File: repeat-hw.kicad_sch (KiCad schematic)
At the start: 39 parts, among them J1 USB_C_Receptacle_USB2.0, U1 nRF5340-QKxx, U2 USBLC6-2SC6, Y1 32MHz

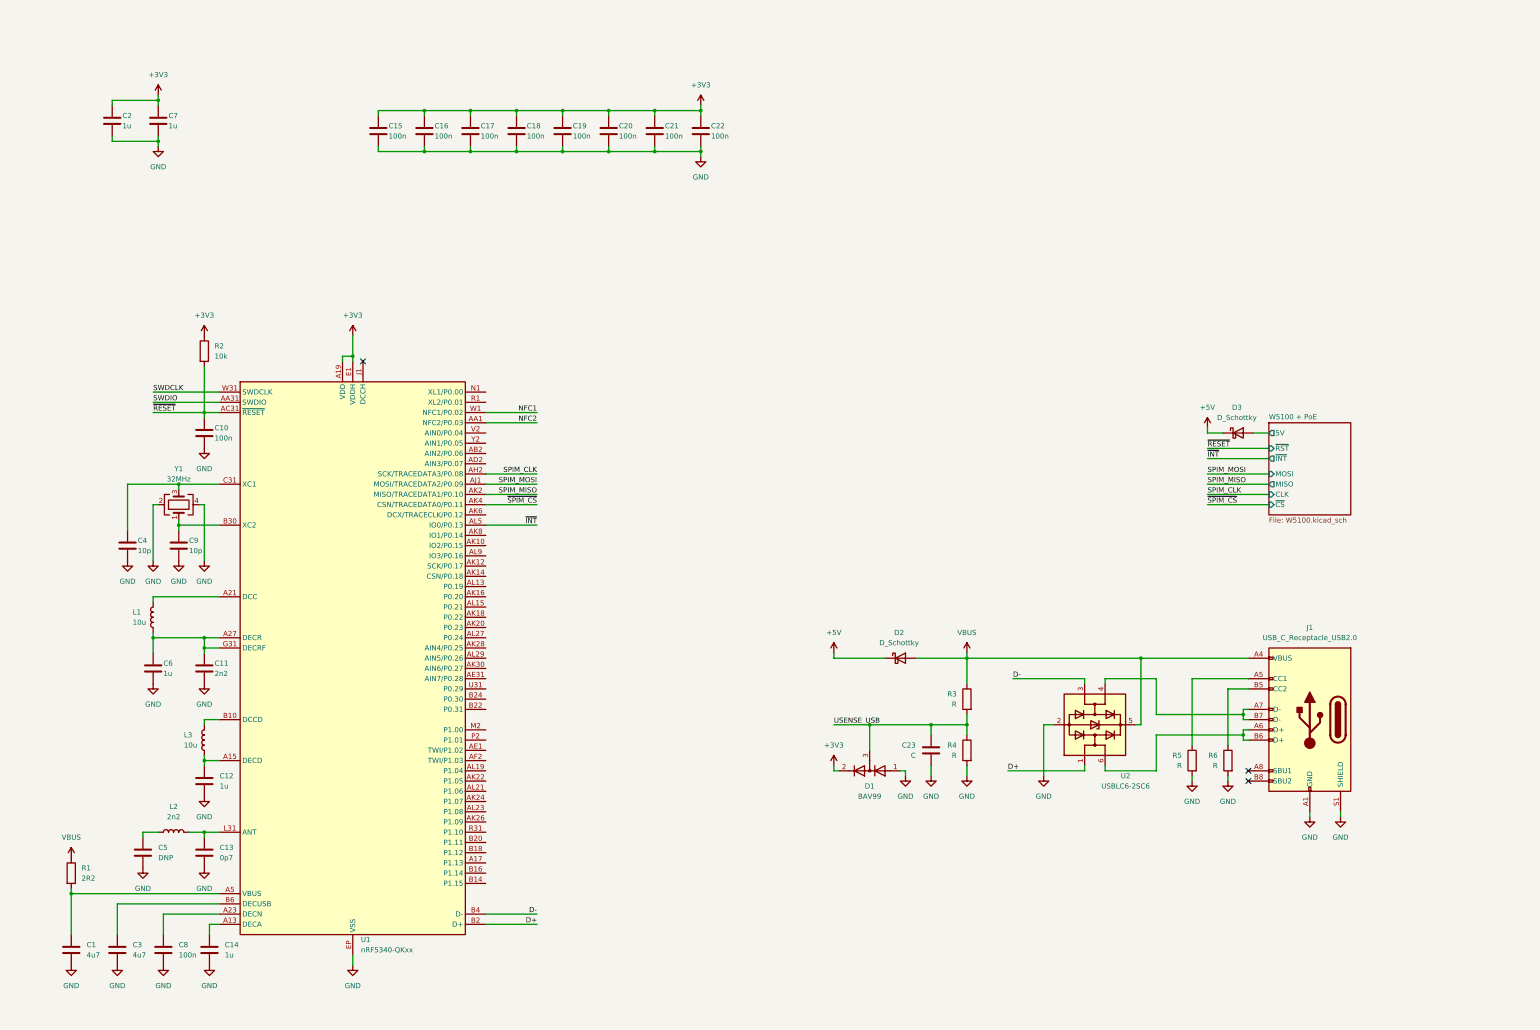
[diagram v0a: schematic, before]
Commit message: Polished schematic
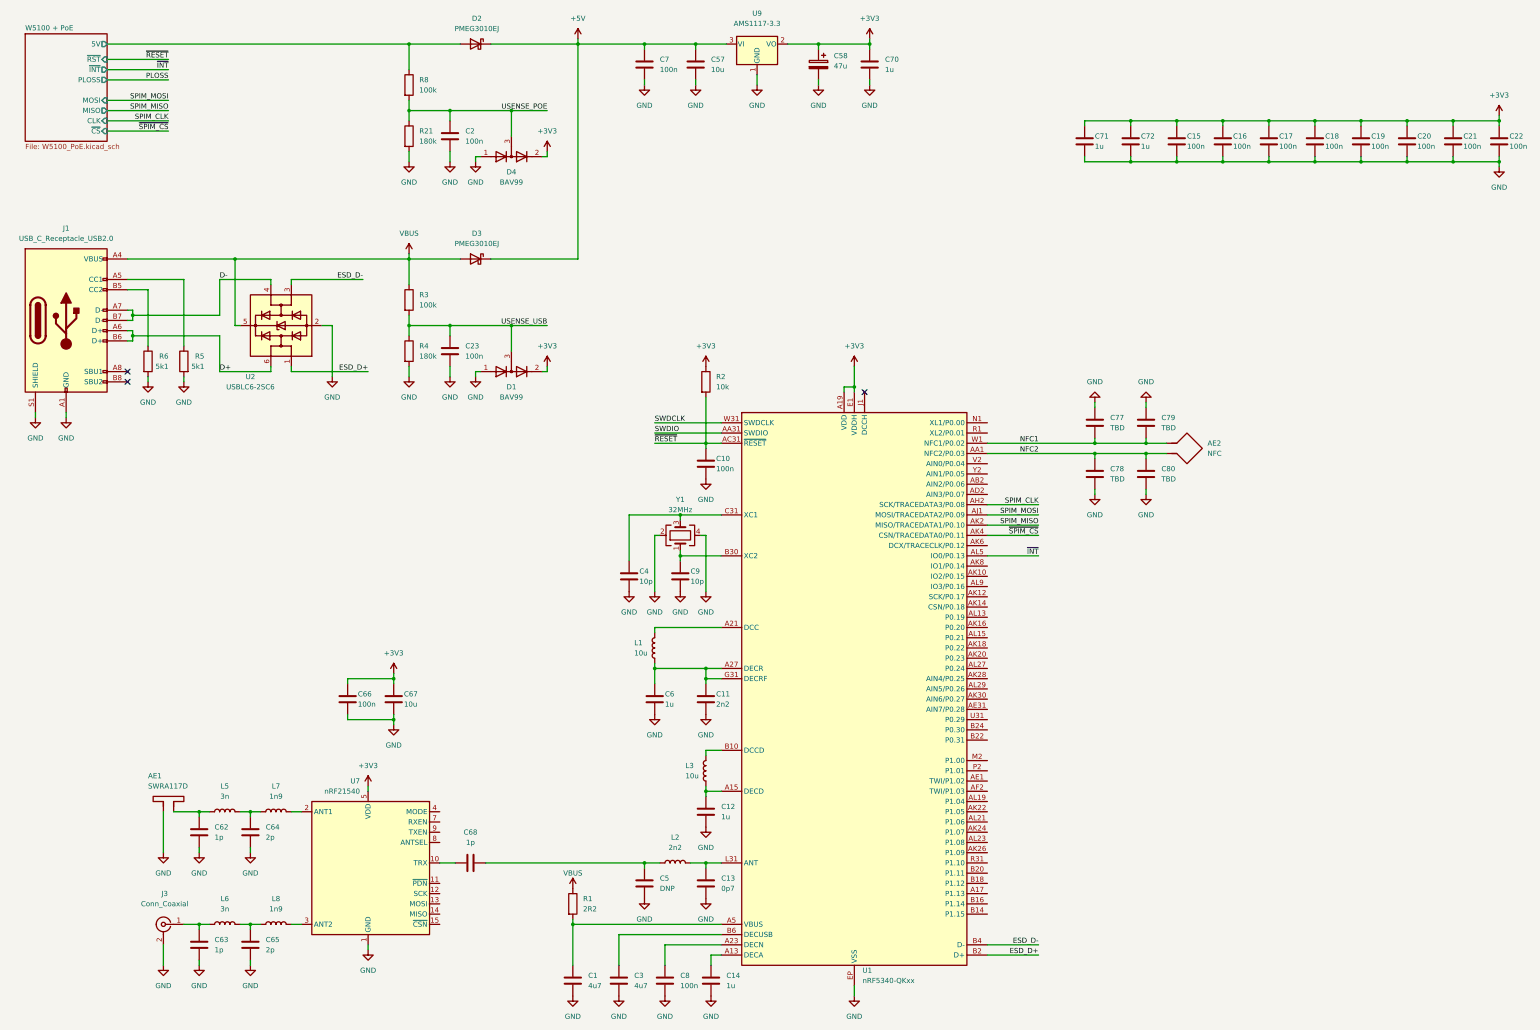
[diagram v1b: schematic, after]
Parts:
- removed D2, D3: D_Schottky, symbol Device:D_Schottky
- added AE1: SWRA117D, RF_Antenna:Texas_SWRA117D_2.4GHz_Left, symbol Device:Antenna_Dipole
- added AE2: NFC, symbol Device:Antenna_Loop
- added C57: 10u, Capacitor_SMD:C_0603_1608Metric, symbol Device:C
- added C58: 47u, symbol Device:C_Polarized
- added C62, C63, C68: 1p, Capacitor_SMD:C_0402_1005Metric, symbol Device:C
- added C64, C65: 2p, Capacitor_SMD:C_0402_1005Metric, symbol Device:C
- added C66: 100n, Capacitor_SMD:C_0402_1005Metric, symbol Device:C
- added C67: 10u, Capacitor_SMD:C_0402_1005Metric, symbol Device:C
- added C70, C71, C72: 1u, Capacitor_SMD:C_0603_1608Metric, symbol Device:C
- added C77, C78, C79, C80: TBD, symbol Device:C
- added D2, D3: PMEG3010EJ, Diode_SMD:D_SOD-323F, symbol Diode:PMEG3010EJ
- added D4: BAV99, Package_TO_SOT_SMD:SOT-23, symbol Diode:BAV99
- added J3: Conn_Coaxial, Connector_Coaxial:U.FL_Hirose_U.FL-R-SMT-1_Vertical, symbol Connector:Conn_Coaxial
- added L5, L6: 3n, Capacitor_SMD:C_0402_1005Metric, symbol Device:L
- added L7, L8: 1n9, Capacitor_SMD:C_0402_1005Metric, symbol Device:L
- added R21: 180k, Resistor_SMD:R_0402_1005Metric, symbol Device:R
- added R8: 100k, Resistor_SMD:R_0402_1005Metric, symbol Device:R
- added U7: nRF21540, Package_DFN_QFN:QFN-16-1EP_4x4mm_P0.65mm_EP2.7x2.7mm_ThermalVias, symbol nordic:nRF21540
- added U9: AMS1117-3.3, Package_TO_SOT_SMD:SOT-223-3_TabPin2, symbol Regulator_Linear:AMS1117-3.3
- C1: footprint Connector_RJ:RJ45_Cetus_J1B1211CCD_Horizontal -> Capacitor_SMD:C_0603_1608Metric
- C12, C14, C3, C6: footprint (none) -> Capacitor_SMD:C_0603_1608Metric
- C2: value 1u -> 100n
- C23: value C -> 100n; footprint (none) -> Capacitor_SMD:C_0402_1005Metric
- C5: footprint (none) -> Capacitor_SMD:C_0402_1005Metric
- C7: value 1u -> 100n; footprint (none) -> Capacitor_SMD:C_0402_1005Metric
- R3: value R -> 100k
- R4: value R -> 180k
- R5, R6: value R -> 5k1
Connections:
- net +3V3: now also C58.1, C66.1, C67.1, C70.1, C71.1, C72.1, D4.2 (A), U7.5 (VDD), U7.6 (VDD), U9.2 (VO); no longer C2.1, C7.1
- net +5V: now also C7.1, C57.1, D2.1 (K), D3.1 (K), U9.3 (VI)
- net D+: now also J1.A6 (D+), J1.B6 (D+), U2.6 (I/O1); no longer U1.B2 (D+), U2.1 (I/O1)
- net D-: now also J1.A7 (D-), J1.B7 (D-), U2.4 (I/O2); no longer U1.B4 (D-), U2.3 (I/O2)
- net GND: now also AE1.1, C57.2, C58.2, C62.2, C63.2, C64.2, C65.2, C66.2, C67.2, C70.2, C71.2, C72.2, C77.1, C78.2, C79.1, C80.2, D4.1 (K), J3.2 (Ext), R21.2, U7.1 (GND), U7.16 (GND), U7.17 (GND), U9.1 (GND)
- net NFC1: now also AE2.1, C77.2, C79.2
- net NFC2: now also AE2.2, C78.1, C80.1
- net VBUS: now also D3.2 (A)
- net W5100 + PoE/5V: now also D2.2 (A), R8.1
- net at C5.1, L2.1: now also C68.2
- new net: C68.1, U7.10 (TRX)
- new net: L7.2, U7.2 (ANT1)
- new net: L8.2, U7.3 (ANT2)
- new net: AE1.2, C62.1, L5.1
- new net: C63.1, J3.1 (In), L6.1
- new net: C64.1, L5.2, L7.1
- new net: C65.1, L6.2, L8.1
- new net ESD_D+: U1.B2 (D+), U2.1 (I/O1)
- new net ESD_D-: U1.B4 (D-), U2.3 (I/O2)
- new net USENSE_POE: C2.1, D4.3 (K), R21.1, R8.2
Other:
- sheet W5100 + PoE: file W5100.kicad_sch -> W5100_PoE.kicad_sch
- sheet W5100 + PoE ports: added PLOSS; removed none
- moved on the sheet: C1, C10, C11, C12, C13, C14, C15, C16, C17, C18, C19, C20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
